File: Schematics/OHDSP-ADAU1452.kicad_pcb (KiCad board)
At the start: 4 copper layers, 100 x 100 mm, 305 parts, among them CN201 COAX, CN401 COAX, CN402 COAX, CN405 COAX, CN406 COAX, P201 CONN_2x1, P203 CONN_6X2, P204 CONN_6x1, P301 CONN_2x1, P302 CONN_2x1, P303 PIN, P304 PIN, P305 PIN, P306 PIN, P601 CONN_02X05, P602 CONN_02X05, P603 CONN_02X05, P604 CONN_02X05, P605 CONN_3x1, P606 CONN_6X2, P607 CONN_02X05, P608 CONN_02X05, P609 CONN_02X20, P610 CONN_02X05, P611 CONN_5x1, P613 CONN_02X05, P614 CONN_02X05, P615 CONN_02X05, P616 CONN_02X05, SW202 SWITCH, U201 ADAU1452WBCPZ, U202 ADM13307-5ARZ, U203 25AA1024, U301 IC-REG-XRP7659ISTR-F, U302 IC-REG-XRP7659ISTR-F, U304 IC-REG-XC6210B332MR, U305 IC-REG-XC6210B332MR, U401 NB3L553, U501 IC-SPDIF-RX-OPTO, U502 IC-SPDIF-TX-OPTO, X201 24M576

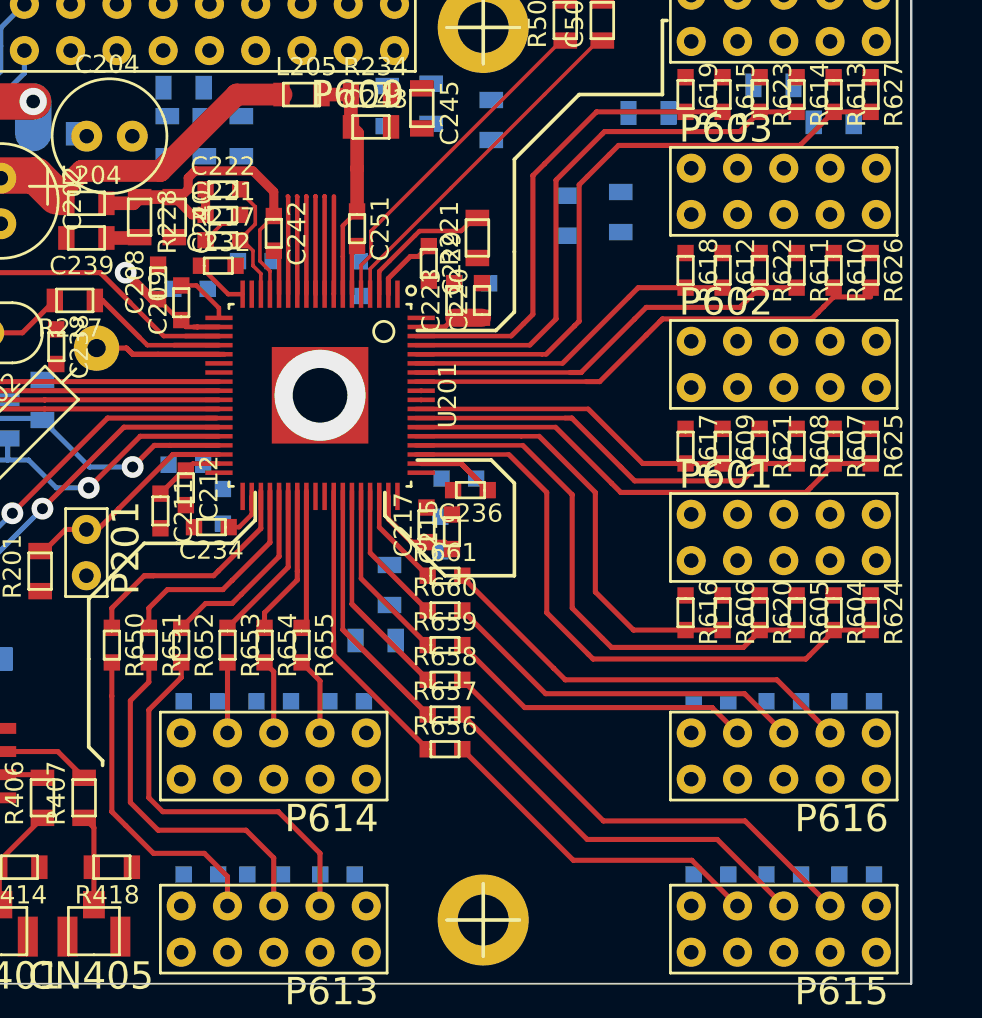
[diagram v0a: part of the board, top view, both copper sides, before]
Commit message: PCB Work
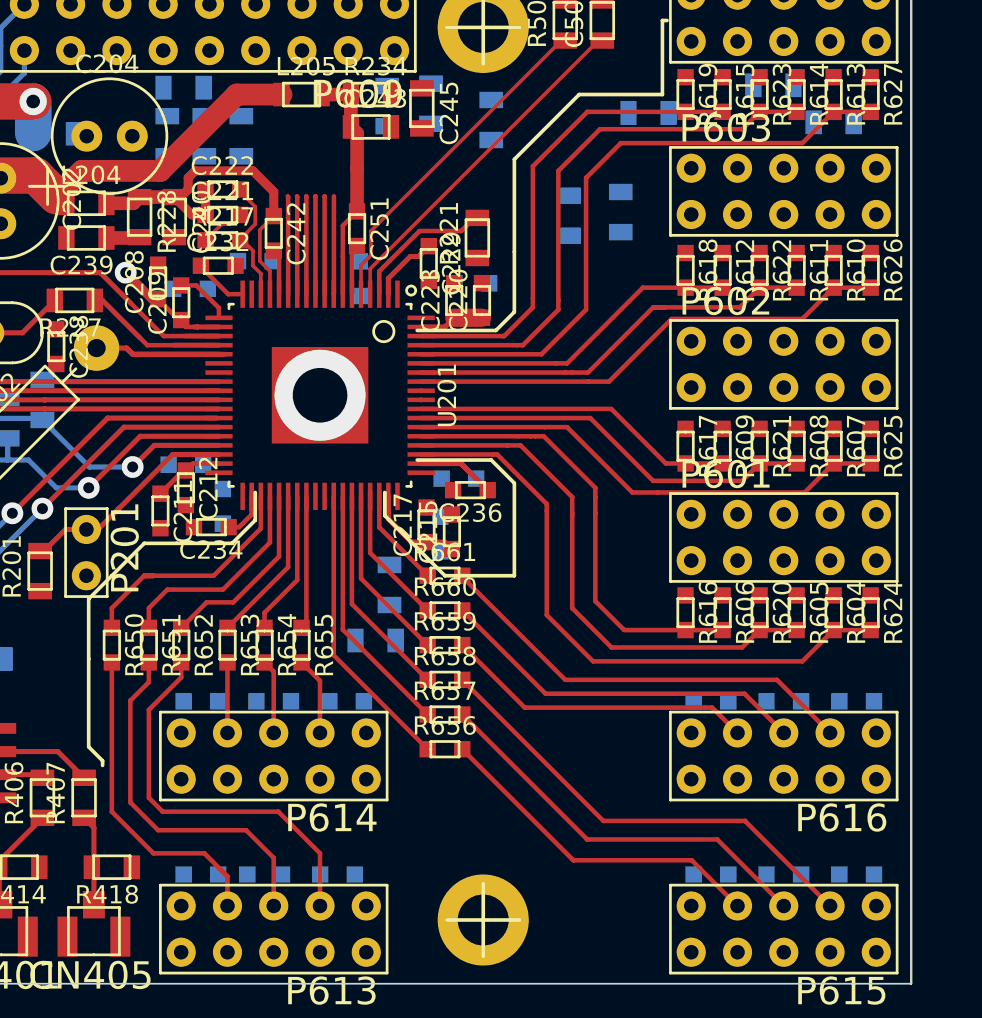
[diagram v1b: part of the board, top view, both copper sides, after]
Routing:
- net /ADAU1452/DACOUT_BCLK2: track 20.8 -> 13.9 mm
- net /ADAU1452/DACOUT_SDATA2: track 18.0 -> 11.8 mm
